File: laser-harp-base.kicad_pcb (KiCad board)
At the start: 2 copper layers, 170 x 72 mm, 65 parts, among them J1 BAR_CONN, J2 LASER1, J3 LASER2, J4 LASER3, J5 LASER4, J6 LASER5, J7 LASER6, J8 LASER7, J9 LASER8, Q1 AO3400A, SW1 OCTAVE, SW2 SCALE, U1 ESP32-S3-Zero, U2 LM393, U3 LM393, U4 LM393, U5 LM393, U6 74AHCT1G125

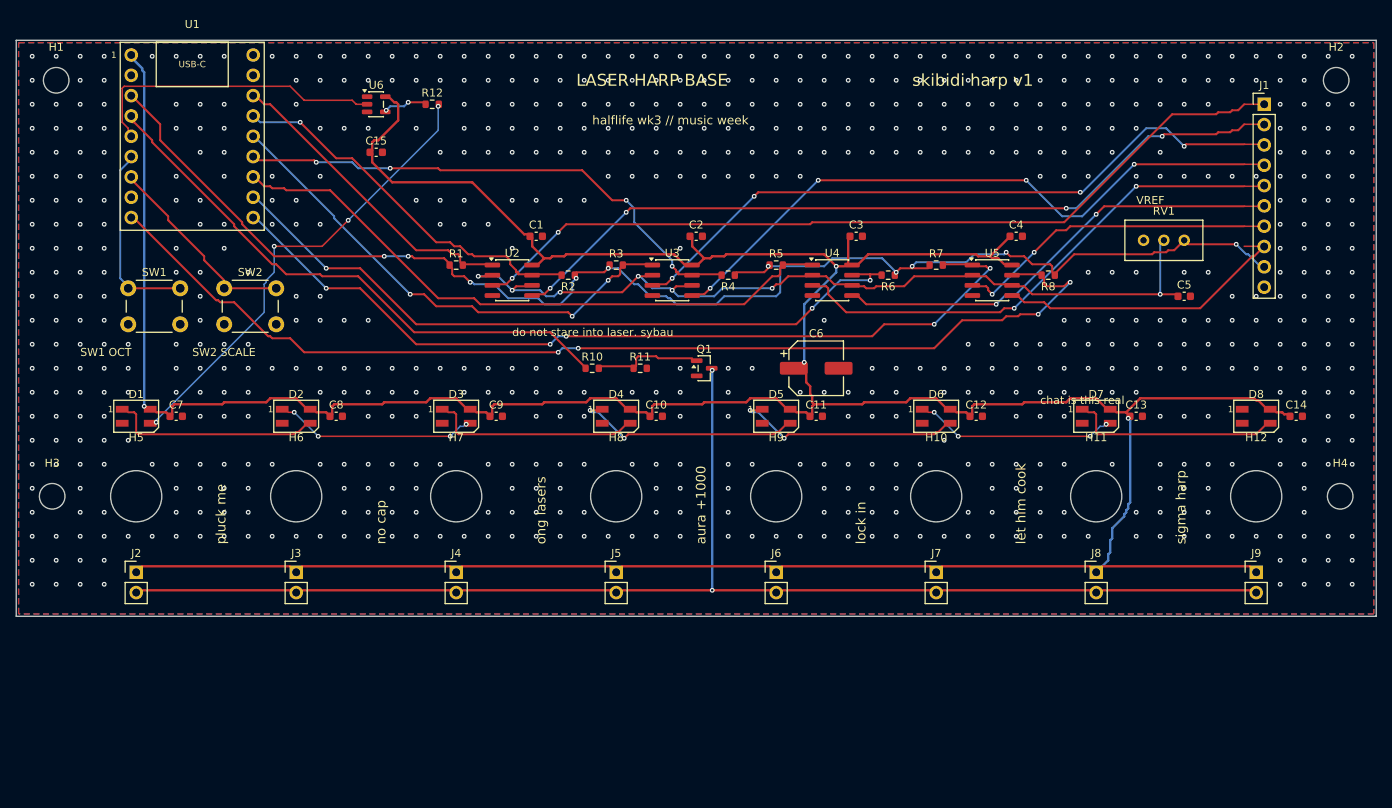
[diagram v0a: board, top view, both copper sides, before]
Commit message: added finishing touches
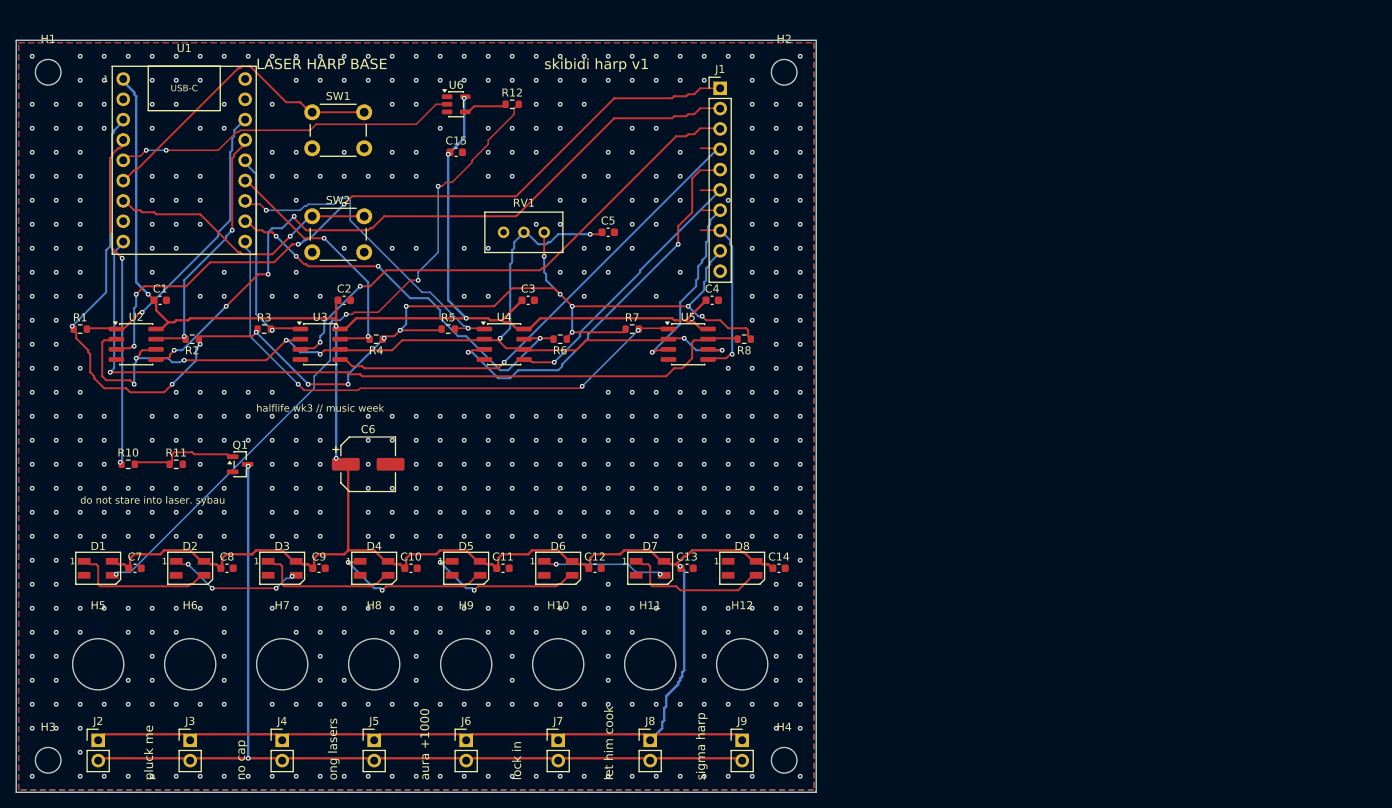
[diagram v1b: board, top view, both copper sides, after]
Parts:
- moved RV1 80.0 mm to (66.0, 24.0)
- moved H4 76.9 mm to (96.0, 90.0)
- moved C5 72.4 mm to (74.0, 24.0)
- moved H2 69.0 mm to (96.0, 4.00)
- moved J1 68.0 mm to (88.0, 6.00)
- moved H12 67.6 mm to (90.8, 78.0)
- moved J9 67.6 mm to (90.8, 87.5)
- moved C14 67.4 mm to (95.3, 66.0)
- moved D8 67.0 mm to (90.8, 66.0)
- moved H11 59.6 mm to (79.2, 78.0)
- moved J8 59.6 mm to (79.2, 87.5)
- moved C13 59.3 mm to (83.8, 66.0)
- moved Q1 59.2 mm to (28.0, 53.0)
- moved R10 59.2 mm to (14.0, 53.0)
- moved R11 59.2 mm to (20.0, 53.0)
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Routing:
- net /+5V: track 455.9 -> 337.3 mm, vias 4 -> 7
- net /LASER_GND: track 157.0 -> 106.5 mm
- net /CMP6: track 88.7 -> 48.8 mm, vias 3 -> 4
- net /CMP8: track 134.3 -> 96.0 mm, vias 4 -> 1
- net /CMP7: track 106.0 -> 68.4 mm, vias 5 -> 3
- net /CMP5: track 76.7 -> 39.1 mm, vias 0 -> 2
- net /CMP3: track 60.2 -> 24.5 mm, vias 3 -> 1
- net /CMP4: track 63.7 -> 29.3 mm, vias 4 -> 2
- net /LASER_EN: track 69.4 -> 41.0 mm, vias 0 -> 2
- net /NEO0: track 57.6 -> 84.3 mm
- net /SENS6: track 56.2 -> 35.0 mm, vias 2 -> 1
- net /SENS4: track 81.2 -> 60.1 mm, vias 4 -> 1
- net /SENS3: track 84.6 -> 64.1 mm, vias 4 -> 2
- net /SENS8: track 36.4 -> 20.4 mm, vias 0 -> 1
- net /SENS7: track 39.6 -> 24.4 mm, vias 2 -> 1
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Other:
- board size 170 x 72 mm -> 100 x 94 mm
- board text removed: "SW1 OCT"
- board text removed: "SW2 SCALE"
- board text removed: "VREF"
- board text removed: "chat is this real"
